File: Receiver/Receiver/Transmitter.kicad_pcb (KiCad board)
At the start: 4 copper layers, 44.6 x 98.5 mm, 56 parts, among them J1 SSW-104-01-T-D-LL, J10 Conn_01x03, J11 Conn_01x03, J12 Conn_01x03, J13 Conn_01x03, J14 Conn_01x03, J2 105-1103-001, J3 Conn_01x06, J4 105-1103-001, J5 105-1103-001, J8 FCR7350R, J9 FCR7350R, Q1 RJF0408JPD-01#J3, Q10 RJF0408JPD-01#J3, Q3 RJF0408JPD-01#J3, Q5 RJF0408JPD-01#J3, Q6 RJF0408JPD-01#J3, Q9 RJF0408JPD-01#J3, SW1 D6R90F2LFS, SW2 500SSP1S2M2QEA, U1 ANT13SECQE, U2 STM32F030R8Tx, U3 MIC5205-3.3YM5, U4 TPS565201DDCR, U7 HEF4104BT_653

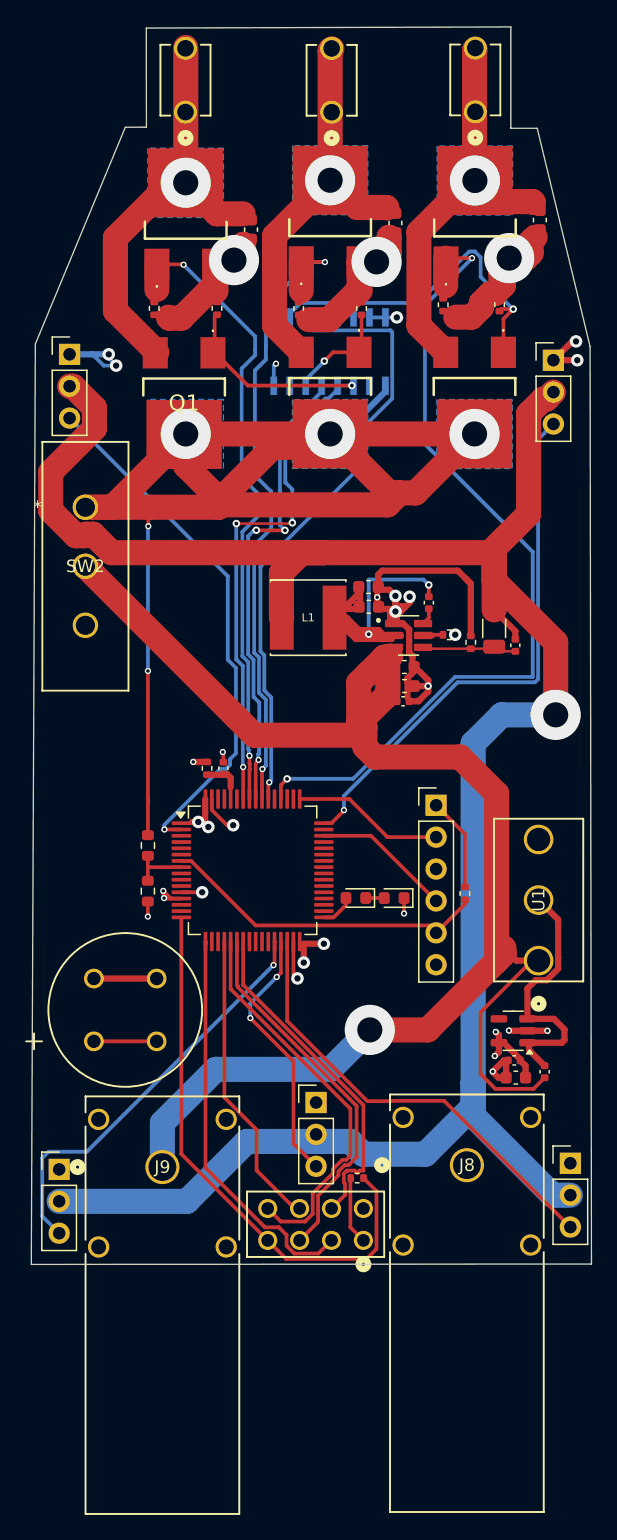
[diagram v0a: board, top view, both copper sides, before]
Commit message: V2 PCB
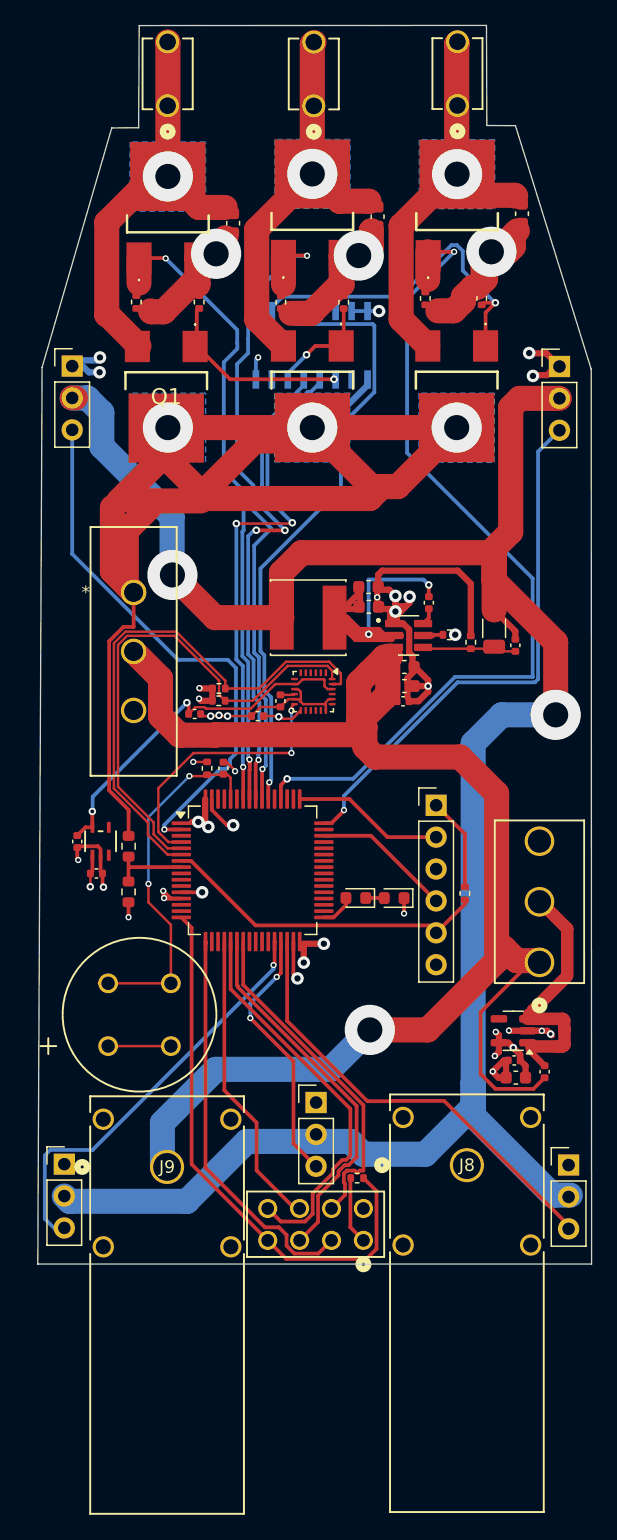
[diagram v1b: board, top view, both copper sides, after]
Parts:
- added C15: 1uF, Capacitor_SMD:C_0402_1005Metric, F.Cu at (100.2, 79.3)
- added C16: 0.1uF, Capacitor_SMD:C_0402_1005Metric, F.Cu at (107.0, 78.3)
- added C17: 0.1uF, Capacitor_SMD:C_0402_1005Metric, F.Cu at (90.9, 89.5)
- added C18: 1uF, Capacitor_SMD:C_0402_1005Metric, F.Cu at (92.4, 92.0)
- added C3: 1uF, Capacitor_SMD:C_0402_1005Metric, F.Cu at (105.2, 79.5)
- added R15: 10k, Resistor_SMD:R_0402_1005Metric, F.Cu at (102.1, 77.3)
- added R16: 10k, Resistor_SMD:R_0402_1005Metric, F.Cu at (102.1, 78.2)
- added U5: ICM-20948, Sensor_Motion:InvenSense_QFN-24_3x3mm_P0.4mm, F.Cu at (109.7, 77.5)
- added U8: MIC5365-1.8YC5-TR, Libary1:SC-70_C5_MCH, F.Cu at (92.7, 89.4)
- moved SW2 7.79 mm to (95.3, 69.6)
- moved R14 1.54 mm to (94.9, 93.5)
- moved R13 1.54 mm to (95.0, 89.8)
- moved C10 1.51 mm to (126.3, 39.5)
- moved C8 1.51 mm to (103.3, 40.2)
- moved C9 1.51 mm to (114.8, 39.7)
- moved J2 1.51 mm to (98.1, 30.9)
- moved J5 1.51 mm to (121.1, 30.8)
- moved Q1 1.51 mm to (97.9, 54.8)
- moved Q10 1.51 mm to (121.1, 38.0)
- moved J4 1.51 mm to (109.7, 30.9)
- moved Q3 1.51 mm to (98.1, 38.2)
- moved Q6 1.51 mm to (109.6, 38.0)
- moved R12 1.51 mm to (123.1, 46.2)
- moved R4 1.51 mm to (100.6, 46.5)
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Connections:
- U2 pad 4: unconnected-(U2-PC15-Pad4) -> INT_sense
- U2 pad 5: unconnected-(U2-PF0-Pad5) -> IC21_SDA
- U2 pad 6: unconnected-(U2-PF1-Pad6) -> IC21_SCL
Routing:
- net IC21_SCL: track 0.00 -> 43.5 mm
- net IC21_SDA: track 0.00 -> 41.1 mm
- net Vddio_sensor: track 0.00 -> 28.7 mm, vias 0 -> 2
- net INT_sense: track 0.00 -> 21.4 mm, vias 0 -> 2
- net Net-(U2-BOOT0): track 7.84 -> 29.2 mm, vias 0 -> 2
- net GND: track 104.8 -> 122.5 mm, vias 22 -> 28
- net +3.3V: track 37.3 -> 47.0 mm, vias 11 -> 16
- net +5V: track 180.4 -> 174.7 mm, vias 1 -> 2
- net Vbatt: track 125.0 -> 119.4 mm
- net VBattSense: track 4.66 -> 6.04 mm
- net LFlap: track 42.2 -> 43.5 mm
- net Net-(U5-REGOUT): track 0.00 -> 1.14 mm
- net S6: track 67.5 -> 68.6 mm
- net S1: track 39.7 -> 40.8 mm
- net S4: track 51.6 -> 52.7 mm
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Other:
- board size 44.6 x 98.5 mm -> 44.1 x 98.6 mm
